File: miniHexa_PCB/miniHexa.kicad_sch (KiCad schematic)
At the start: 16 parts, among them U1 STM32F401RETx, Y1 16Mhz

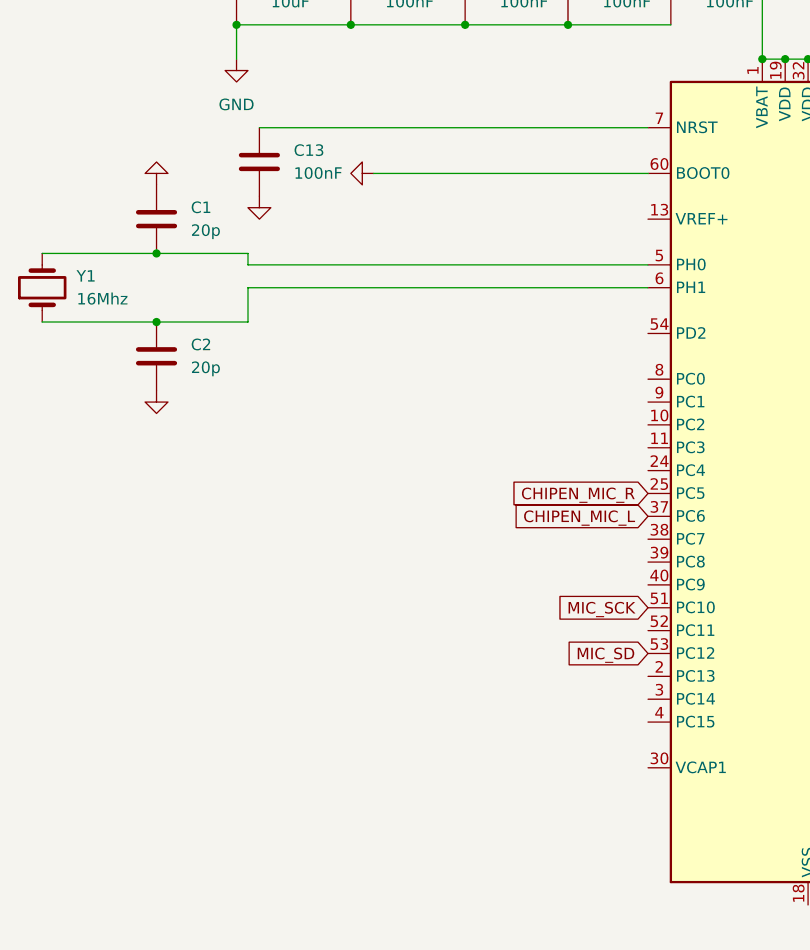
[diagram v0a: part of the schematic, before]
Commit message: update
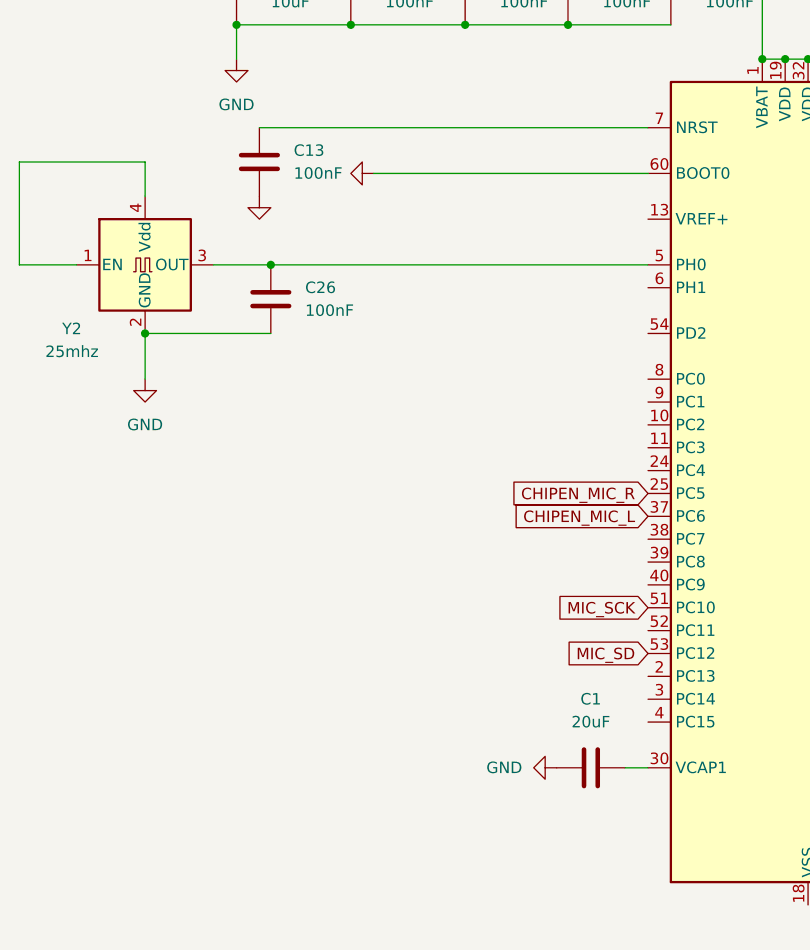
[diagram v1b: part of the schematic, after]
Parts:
- removed C2: 20p, Capacitor_SMD:C_0805_2012Metric, symbol Device:C
- removed Y1: 16Mhz, Crystal:Crystal_HC49-4H_Vertical, symbol Device:Crystal
- added C26: 100nF, Capacitor_SMD:C_0805_2012Metric, symbol Device:C
- added Y2: 25mhz, Oscillator:Oscillator_SMD_Abracon_ASE-4Pin_3.2x2.5mm, symbol Oscillator:ASE-xxxMHz
- C1: value 20p -> 20uF; footprint Capacitor_SMD:C_0805_2012Metric -> (none)
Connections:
- net GND: now also C26.2, Y2.2 (GND)
- net at U1.30 (VCAP1): now also C1.2
- net at U1.5 (PH0): now also C26.1, Y2.3 (OUT); no longer C1.2
- new net: Y2.1 (EN), Y2.4 (Vdd)
